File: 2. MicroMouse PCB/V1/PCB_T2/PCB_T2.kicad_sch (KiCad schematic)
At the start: 17 parts, among them U1 STM32F407VGTx, Y1 48MHz

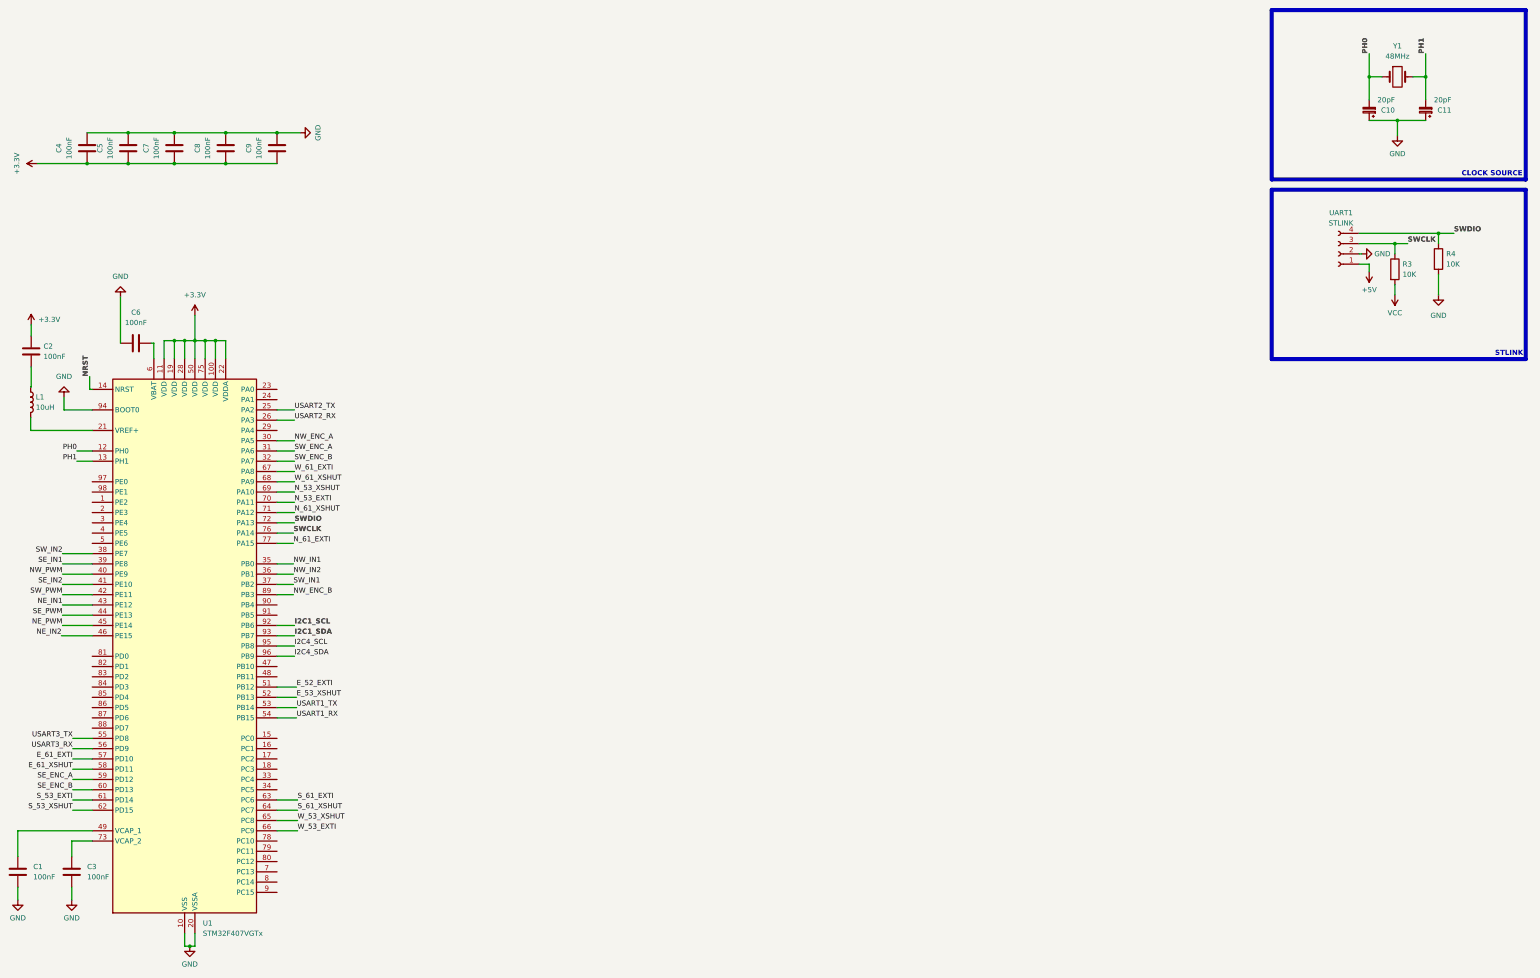
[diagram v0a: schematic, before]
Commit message: update PCB 12/08/2024
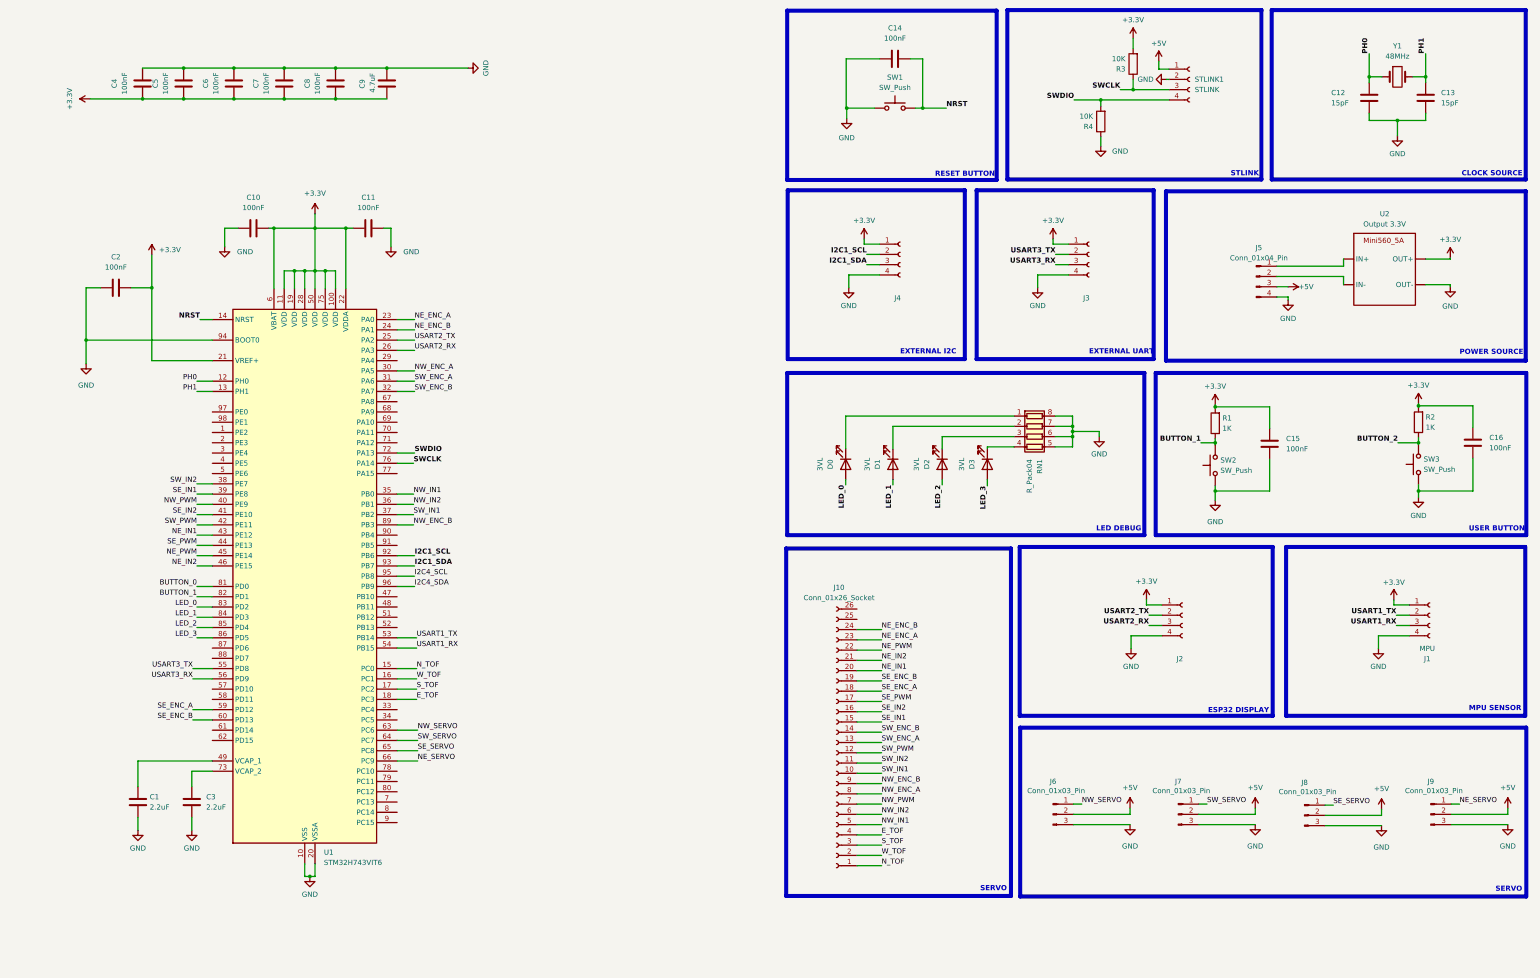
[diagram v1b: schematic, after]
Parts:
- removed C10, C11: 20pF, Capacitor_SMD:C_0603_1608Metric, symbol Device:C_Polarized_Small
- removed L1: 10uH, Capacitor_SMD:C_0805_2012Metric_Pad1.18x1.45mm_HandSolder, symbol Device:L
- added C10, C11, C14, C15, C16: 100nF, Capacitor_SMD:C_0402_1005Metric, symbol Device:C
- added C12, C13: 15pF, Capacitor_SMD:C_0402_1005Metric, symbol Device:C
- added D0, D1, D2, D3: 3VL, LED_SMD:LED_0603_1608Metric, symbol Device:LED
- added J1: MPU, Connector_PinHeader_2.54mm:PinHeader_1x04_P2.54mm_Vertical, symbol Connector:Conn_01x04_Socket
- added J10: Conn_01x26_Socket, Connector_FFC-FPC:Hirose_FH12-26S-0.5SH_1x26-1MP_P0.50mm_Horizontal, symbol Connector:Conn_01x26_Socket
- added J2, J3, J4: MPU, Connector_JST:JST_SH_BM04B-SRSS-TB_1x04-1MP_P1.00mm_Vertical, symbol Connector:Conn_01x04_Socket
- added J5: Conn_01x04_Pin, symbol Connector:Conn_01x04_Pin
- added J6, J7, J8, J9: Conn_01x03_Pin, Connector_JST:JST_SH_BM03B-SRSS-TB_1x03-1MP_P1.00mm_Vertical, symbol Connector:Conn_01x03_Pin
- added R1, R2: 1K, Resistor_SMD:R_0402_1005Metric, symbol Device:R
- added RN1: R_Pack04, Resistor_SMD:R_Array_Convex_4x0603, symbol Device:R_Pack04
- added SW1, SW2, SW3: SW_Push, Button_Switch_SMD:SW_Tactile_SPST_NO_Straight_CK_PTS636Sx25SMTRLFS, symbol Switch:SW_Push
- added U2: Output 3.3V, Mini560:Mini560_5A, symbol Mini560-5A:Mini560-5A
- C1, C3: value 100nF -> 2.2uF; footprint Capacitor_SMD:C_0603_1608Metric -> Capacitor_Tantalum_SMD:CP_EIA-3216-10_Kemet-I
- C2, C4, C5, C6, C7, C8: footprint Capacitor_SMD:C_0603_1608Metric -> Capacitor_SMD:C_0402_1005Metric
- C9: value 100nF -> 4.7uF; footprint Capacitor_SMD:C_0603_1608Metric -> Capacitor_Tantalum_SMD:CP_EIA-3216-10_Kemet-I
- R3, R4: footprint Resistor_SMD:R_0603_1608Metric -> Resistor_SMD:R_0402_1005Metric
- STLINK1: renamed from UART1; footprint JST254:JST 4 -> Connector_JST:JST_SH_SM04B-SRSS-TB_1x04-1MP_P1.00mm_Horizontal
- U1: value STM32F407VGTx -> STM32H743VIT6
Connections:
- net VCC is gone; now on net +3.3V: R3.2
- net +3.3V: now also C2.2, C6.1, U1.21 (VREF+), U1.6 (VBAT), C10.2, C11.1, C15.2, C16.2, J1.1 (Pin_1), J2.1 (Pin_1), J3.1 (Pin_1), J4.1 (Pin_1), R1.2, R2.2, U2. (OUT-); no longer C2.1
- net +5V: now also J5.3 (Pin_3), J6.2 (Pin_2), J7.2 (Pin_2), J8.2 (Pin_2), J9.2 (Pin_2)
- net GND: now also C2.1, C6.2, R4.1, C10.1, C11.2, C12.1, C13.1, C14.1, C15.1, C16.1, J1.4 (Pin_4), J2.4 (Pin_4), J3.4 (Pin_4), J4.4 (Pin_4), J5.4 (Pin_4), J6.3 (Pin_3), J7.3 (Pin_3), J8.3 (Pin_3), J9.3 (Pin_3), RN1.5 (R4.2), RN1.6 (R3.2), RN1.7 (R2.2), RN1.8 (R1.2), SW1.1, SW2.1, SW3.1, U2. (OUT-); no longer C6.1, R4.2
- net I2C1_SCL: now also J4.2 (Pin_2)
- net I2C1_SDA: now also J4.3 (Pin_3)
- net NE_IN1: now also J10.20 (Pin_20)
- net NE_IN2: now also J10.21 (Pin_21)
- net NE_PWM: now also J10.22 (Pin_22)
- net NRST: now also C14.2, SW1.2
- net NW_ENC_A: now also J10.8 (Pin_8)
- net NW_ENC_B: now also J10.9 (Pin_9)
- net NW_IN1: now also J10.5 (Pin_5)
- net NW_IN2: now also J10.6 (Pin_6)
- net NW_PWM: now also J10.7 (Pin_7)
- net PH0: now also C12.2
- net PH1: now also C13.2
- net SE_ENC_A: now also J10.18 (Pin_18)
- net SE_ENC_B: now also J10.19 (Pin_19)
- net SE_IN1: now also J10.15 (Pin_15)
- net SE_IN2: now also J10.16 (Pin_16)
- net SE_PWM: now also J10.17 (Pin_17)
- net SWDIO: now also R4.2; no longer R4.1
- net SW_ENC_A: now also J10.13 (Pin_13)
- net SW_ENC_B: now also J10.14 (Pin_14)
- net SW_IN1: now also J10.10 (Pin_10)
- net SW_IN2: now also J10.11 (Pin_11)
- net SW_PWM: now also J10.12 (Pin_12)
- net USART1_RX: now also J1.3 (Pin_3)
- net USART1_TX: now also J1.2 (Pin_2)
- net USART2_RX: now also J2.3 (Pin_3)
- net USART2_TX: now also J2.2 (Pin_2)
- net USART3_RX: now also J3.3 (Pin_3)
- net USART3_TX: now also J3.2 (Pin_2)
- net N_TOF: now reaches U1.15 (PC0)
- net N_TOF: now also J10.1 (Pin_1)
- net W_TOF: now reaches U1.16 (PC1)
- net W_TOF: now also J10.2 (Pin_2)
- net S_TOF: now reaches U1.17 (PC2)
- net S_TOF: now also J10.3 (Pin_3)
- net E_TOF: now reaches U1.18 (PC3)
- net E_TOF: now also J10.4 (Pin_4)
- net NE_ENC_A: now reaches U1.23 (PA0)
- net NE_ENC_A: now also J10.23 (Pin_23)
- net NE_ENC_B: now reaches U1.24 (PA1)
- net NE_ENC_B: now also J10.24 (Pin_24)
- net BUTTON_0: now reaches U1.81 (PD0)
- net BUTTON_1: now reaches U1.82 (PD1)
- net BUTTON_1: now also R1.1, SW2.2
- net LED_0: now reaches U1.83 (PD2)
- net LED_0: now also D0.2 (A)
- net LED_1: now reaches U1.84 (PD3)
- net LED_1: now also D1.2 (A)
- net LED_2: now reaches U1.85 (PD4)
- net LED_2: now also D2.2 (A)
- net LED_3: now reaches U1.86 (PD5)
- net LED_3: now also D3.2 (A)
- net E_52_EXTI: no longer names the net of U1.51 (PB12)
- net E_53_XSHUT: no longer names the net of U1.52 (PB13)
- net E_61_EXTI: no longer names the net of U1.57 (PD10)
- net E_61_XSHUT: no longer names the net of U1.58 (PD11)
- net N_53_EXTI: no longer names the net of U1.70 (PA11)
- net N_53_XSHUT: no longer names the net of U1.69 (PA10)
- net N_61_EXTI: no longer names the net of U1.77 (PA15)
- net N_61_XSHUT: no longer names the net of U1.71 (PA12)
- net S_53_EXTI: no longer names the net of U1.61 (PD14)
- net S_53_XSHUT: no longer names the net of U1.62 (PD15)
- net S_61_EXTI renamed NW_SERVO
- net NW_SERVO: now also J6.1 (Pin_1)
- net S_61_XSHUT renamed SW_SERVO
- net SW_SERVO: now also J7.1 (Pin_1)
- net W_53_EXTI renamed NE_SERVO
- net NE_SERVO: now also J9.1 (Pin_1)
- net W_53_XSHUT renamed SE_SERVO
- net SE_SERVO: now also J8.1 (Pin_1)
- net W_61_EXTI: no longer names the net of U1.67 (PA8)
- net W_61_XSHUT: no longer names the net of U1.68 (PA9)
- new net: D3.1 (K), RN1.4 (R4.1)
- new net: J5.1 (Pin_1), U2. (OUT-)
- new net: J5.2 (Pin_2), U2. (OUT-)
- new net: D0.1 (K), RN1.1 (R1.1)
- new net: D1.1 (K), RN1.2 (R2.1)
- new net: D2.1 (K), RN1.3 (R3.1)
- new net BUTTON_2: R2.1, SW3.2
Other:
- note added: "ESP32 DISPLAY"
- note added: "EXTERNAL I2C"
- note added: "EXTERNAL UART"
- note added: "LED DEBUG"
- note added: "MPU SENSOR"
- note added: "POWER SOURCE"
- note added: "RESET BUTTON"
- note added: "SERVO"
- note added: "USER BUTTON"
- moved on the sheet: C1, C2, C3, C4, C5, C7, C8, C9, R3, R4, STLINK1, U1
